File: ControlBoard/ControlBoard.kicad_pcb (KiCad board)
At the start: 2 copper layers, 144 x 106 mm, 195 parts, among them J1 PowerIn, J10 Conn_01x01, J11 Conn_01x01, J12 Conn_01x01, J13 Conn_01x01, J14 Conn_01x01, J15 Conn_01x01, J16 Conn_01x06, J17 Conn_01x06, J18 Conn_01x06, J19 HALLSENS, J2 UART, J20 Conn_01x06, J21 HALLSENS2, J22 PowerIn, J3 ICSP, J4 MTR1, J5 MTR2, J6 Ultrasonic Transmitter, J7 Ultrasonic Receiver, J8 Conn_01x01, J9 Conn_01x01, Q1 2N3904, Q2 2N3904, SW1 SW_Push, U1 LM358, U10 LMT85, U11 74HC138, U12 4051, U13 4051, U14 74HC14, U2 LM358, U3 LM358, U4 LM358, U5 ATMEGA328P-PU, U6 LM7805_TO220, U7 74HC595, U8 L298D, U9 74HC595, Y1 16MHz

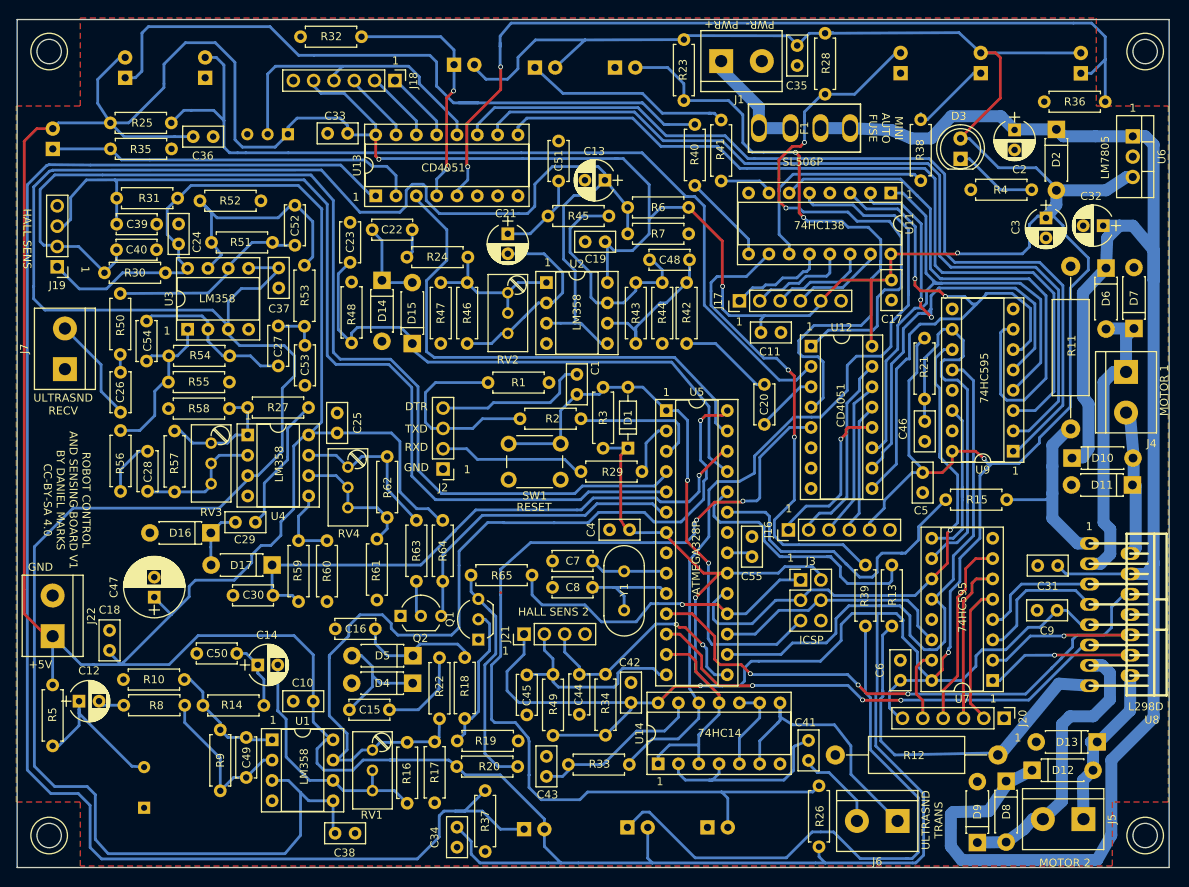
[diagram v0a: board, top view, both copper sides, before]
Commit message: new commit
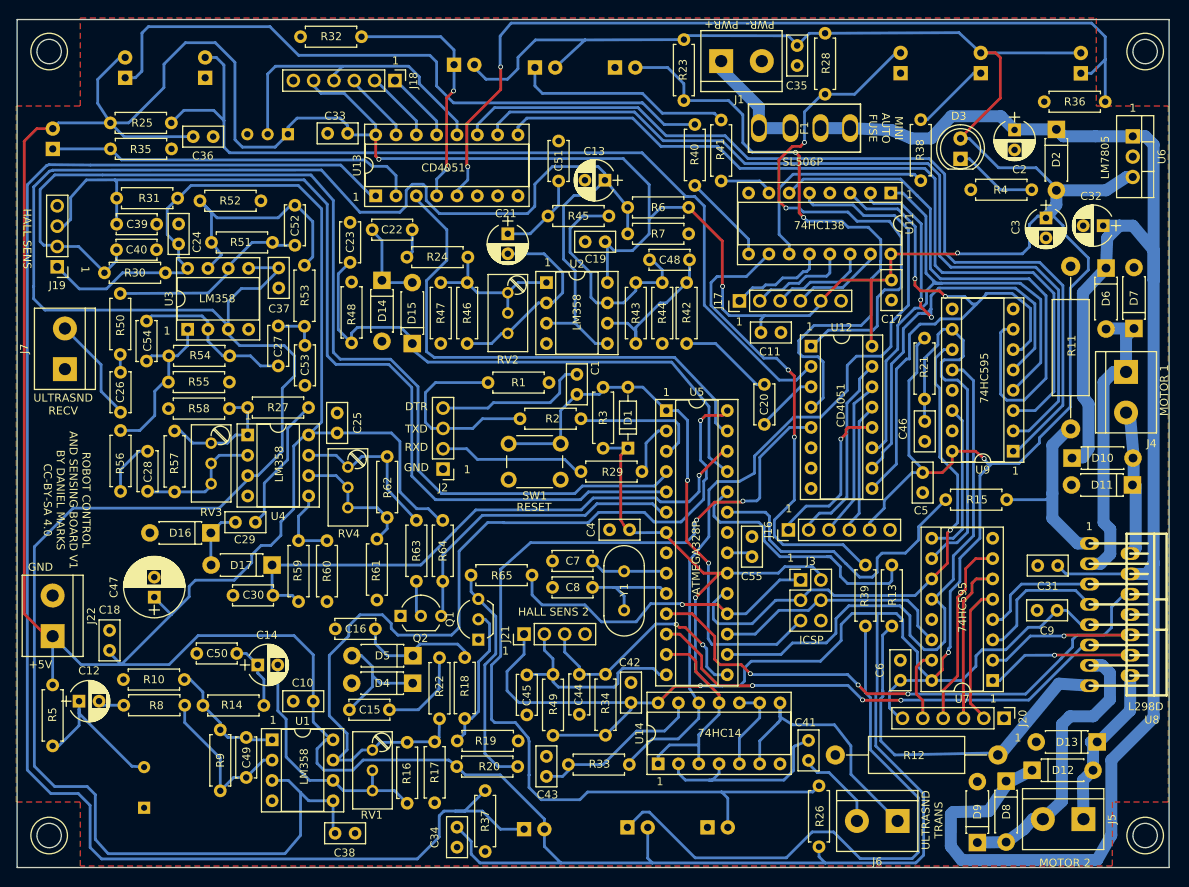
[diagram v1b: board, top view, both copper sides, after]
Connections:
- U9 pad 15: Net-(U9-Pad15) -> unconnected-(U9-QA-Pad15)
- U9 pad 9: Net-(U9-Pad9) -> unconnected-(U9-~{QH}-Pad9)
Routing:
- net +5V: track 1089.6 -> 1074.9 mm
- net Net-(ID3-K): track 86.8 -> 83.5 mm
- net CURSEN1: track 41.2 -> 38.4 mm
- net Net-(J7-Pin_2): track 15.3 -> 13.3 mm
- net SCK: track 69.4 -> 67.5 mm
- net MTRIN2: track 19.1 -> 17.3 mm
- net Net-(J6-Pin_1): track 34.7 -> 32.9 mm
- net Net-(ID1-K): track 11.7 -> 9.91 mm
- net Net-(PT2-C): track 125.0 -> 123.4 mm
- net Net-(PDT4-E): track 33.0 -> 31.4 mm
- net Net-(U7-~{QH}): track 21.2 -> 19.6 mm
- net MTRIN1: track 16.4 -> 15.1 mm
- net Net-(PDT2-E): track 113.1 -> 111.9 mm
- net 2V5: track 326.4 -> 325.3 mm
- net Net-(PT4-C): track 79.9 -> 78.9 mm
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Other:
- net class Default removed
